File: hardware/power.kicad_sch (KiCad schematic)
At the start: 38 parts, among them U1 TLV62569DBV, U2 TLV62569DBV, U3 ECP5U_12_CABGA256, U4 TLV62569DBV, Y1 SITxxxxxx-1x-33E-50.000000

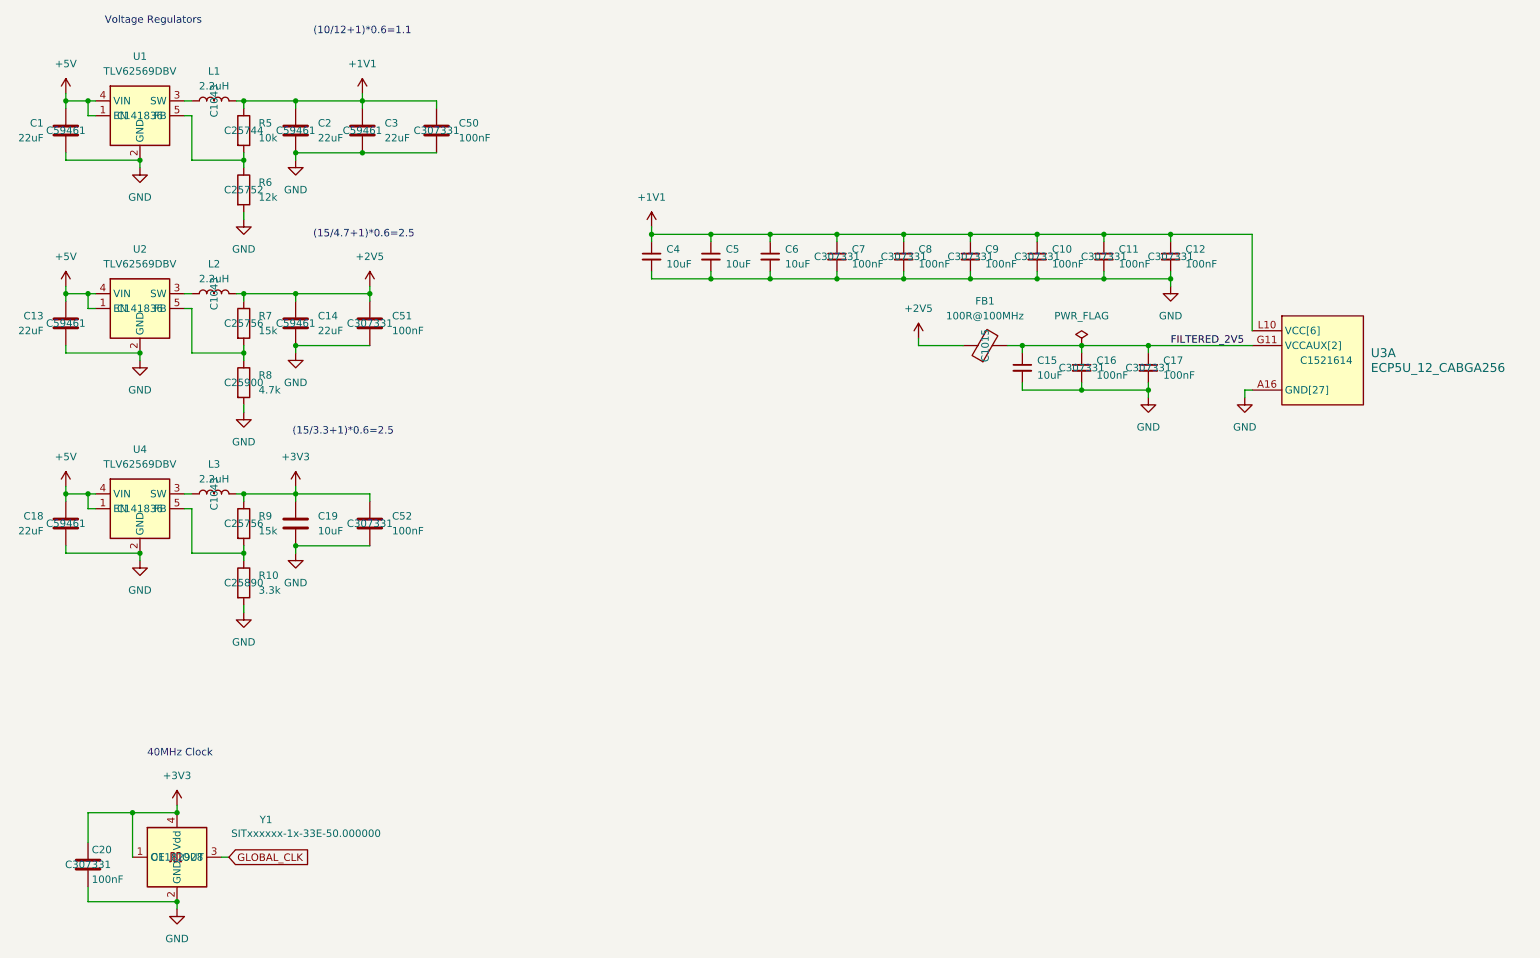
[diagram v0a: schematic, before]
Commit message: Last checks
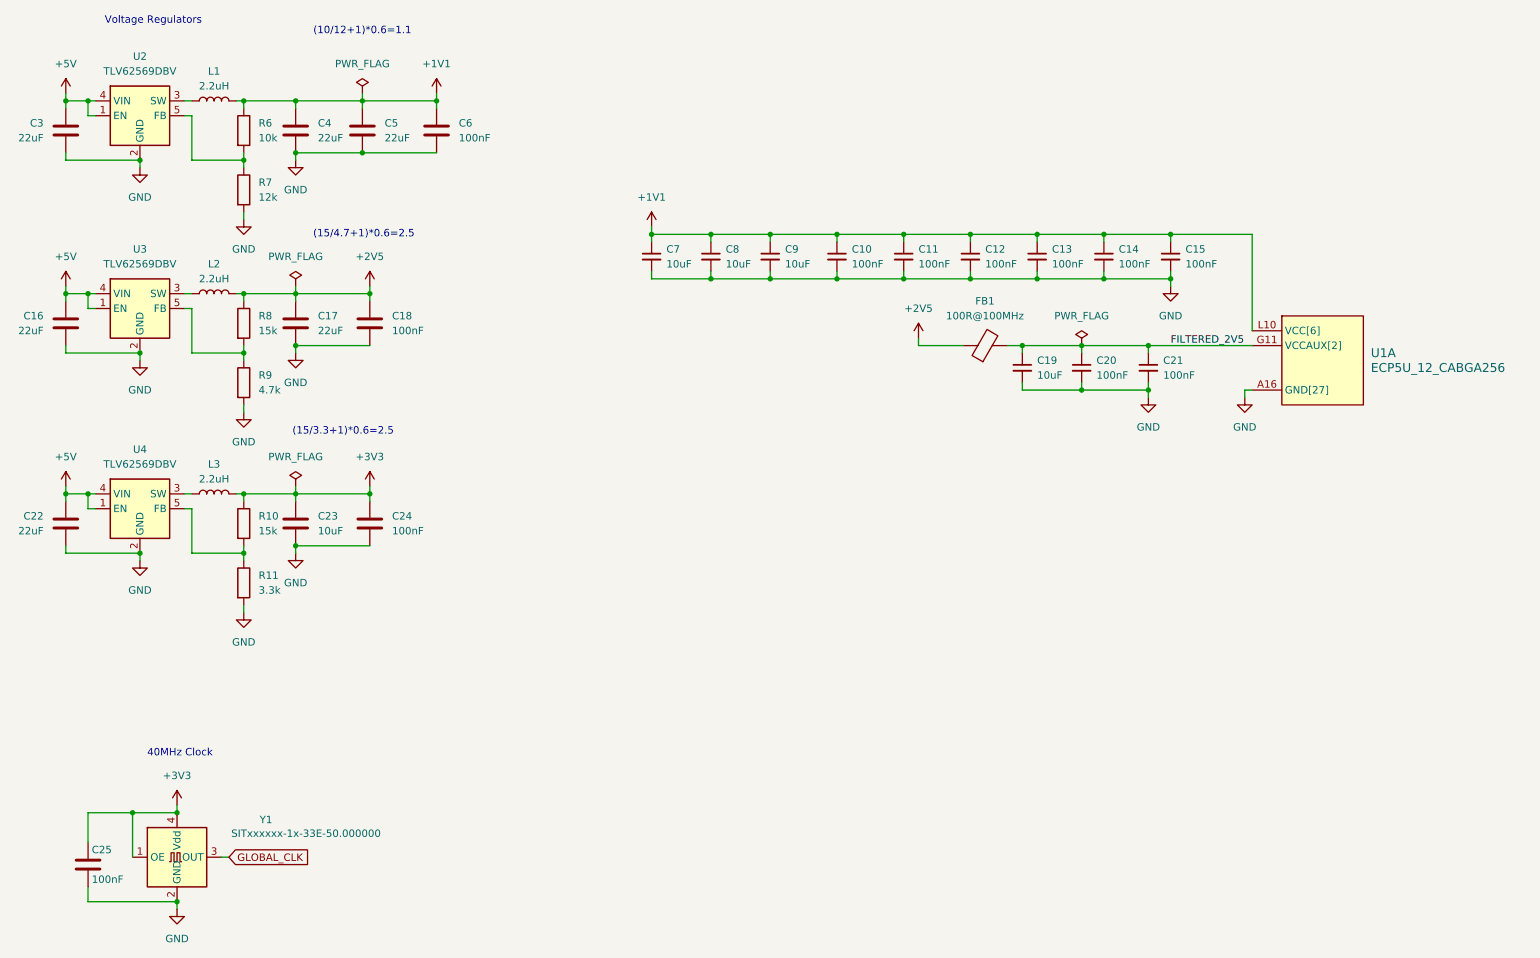
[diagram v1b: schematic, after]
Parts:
- C19: renamed from C15; LCSC Part # (none) -> C19702
- C23: renamed from C19; LCSC Part # (none) -> C19702
- C7: renamed from C4; LCSC Part # (none) -> C19702
- C8: renamed from C5; LCSC Part # (none) -> C19702
- C9: renamed from C6; LCSC Part # (none) -> C19702
- renumbered C7 to C10, C8 to C11, C9 to C12, C10 to C13, C11 to C14, C12 to C15, C13 to C16, C14 to C17, C51 to C18, C16 to C20, C17 to C21, C18 to C22, C52 to C24, C20 to C25, C1 to C3, C2 to C4, C3 to C5, C50 to C6, R9 to R10, R10 to R11, R5 to R6, R6 to R7, R7 to R8, R8 to R9, U3 to U1, U1 to U2, U2 to U3
